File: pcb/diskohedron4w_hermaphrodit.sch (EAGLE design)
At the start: 23 parts, among them IC1 LM2596, U1 SN65LVDS047D, X1 87758-1216, X2 87758-1216

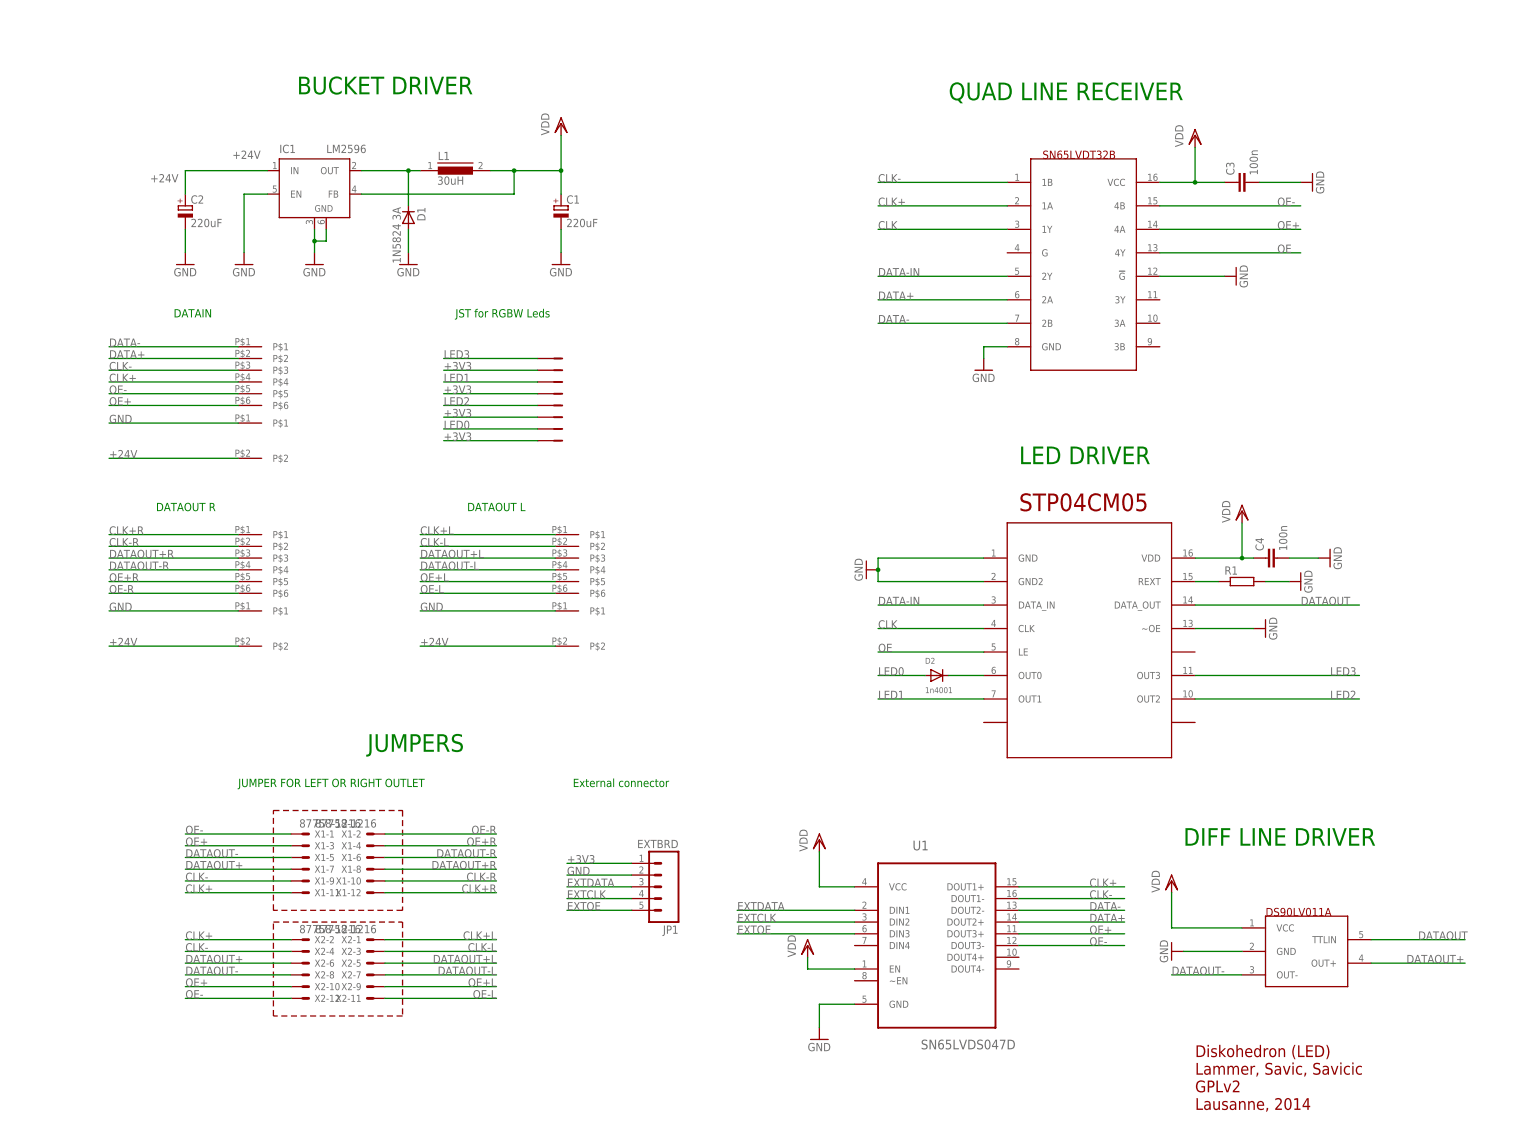
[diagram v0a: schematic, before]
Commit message: last commit before changing physical dimension
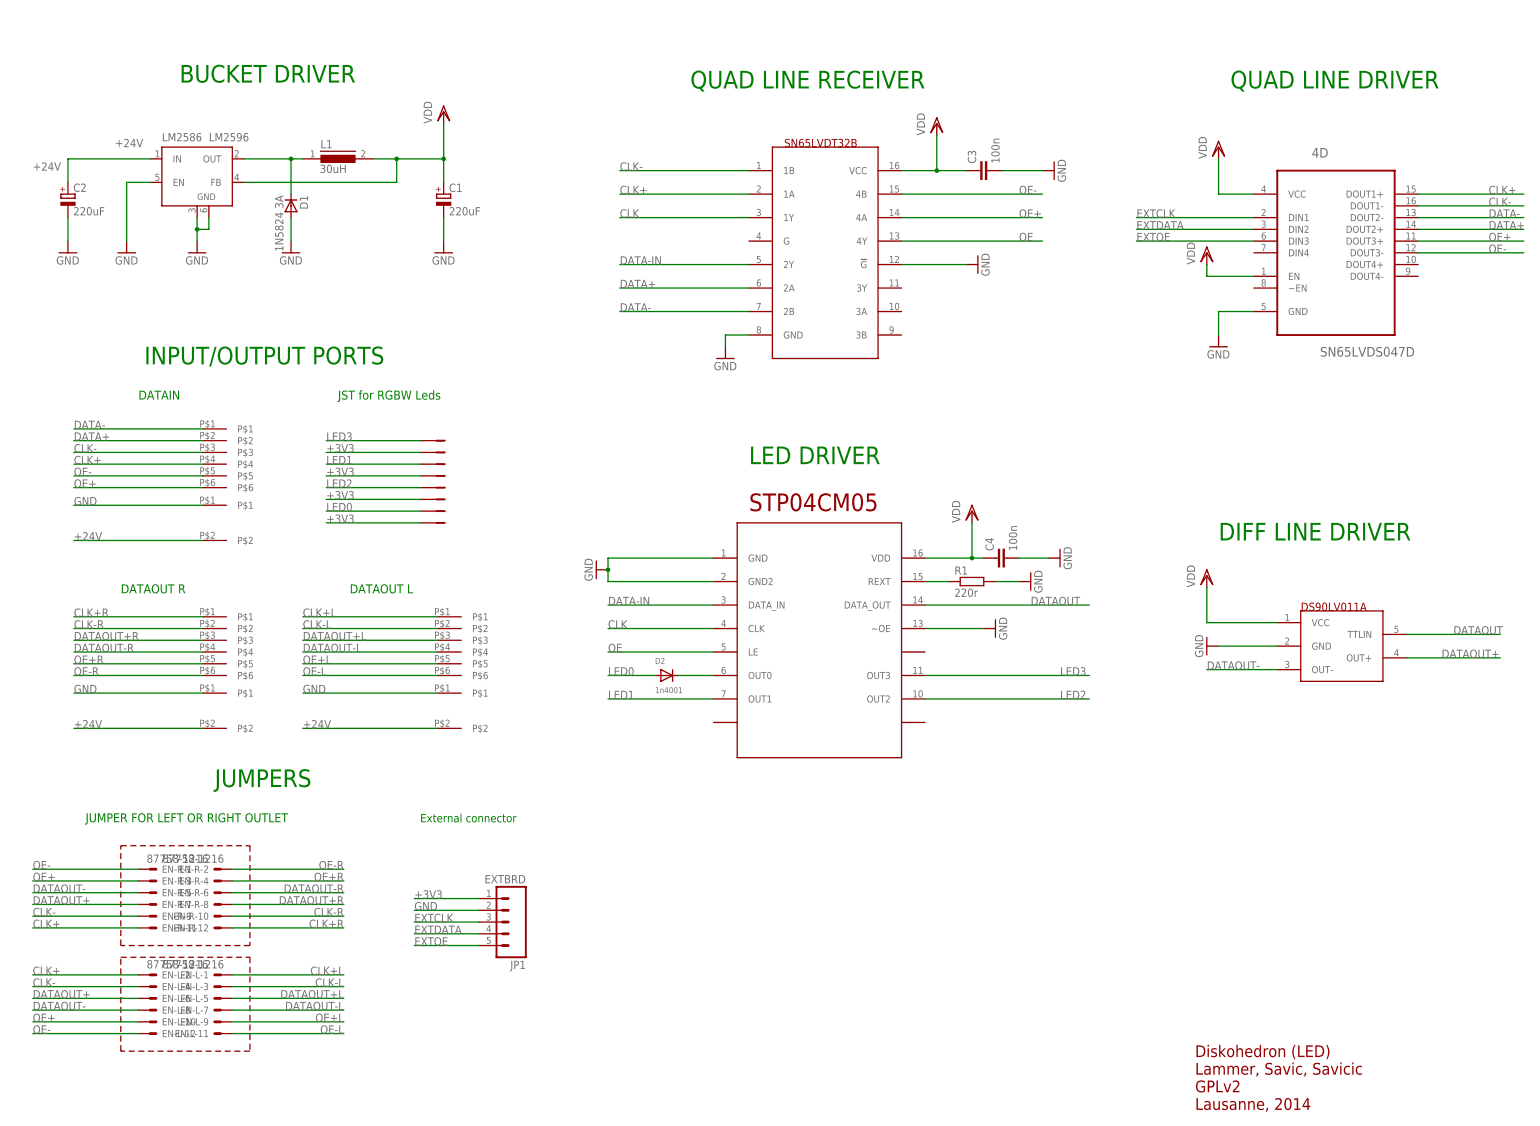
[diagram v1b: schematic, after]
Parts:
- removed IC1: LM2596, linear:LM2596S
- removed U$1: STP04CM05, stp04:STP04CM05
- removed U$11, U$5, U$8: HERMAPHRODITMINI6PIN, diskohedron:HERMAPHRODITMINI6PIN
- removed U$2: SN65LVDST32, diskohedron:SN65LVDST32
- removed U$3: DS90LV011A, diskohedron:DS90LV011A
- removed U$4: 8PIN-ZH, diskohedron:8PIN-ZH
- removed U1: SN65LVDS047D, Texas Instruments_By_element14_Batch_1:SN65LVDS047D
- removed X1, X2: 87758-1216, con-molex:87758-1216
- added 1D: DS90LV011A, diskohedron:DS90LV011A
- added 4D: SN65LVDS047D, Texas Instruments_By_element14_Batch_1:SN65LVDS047D
- added 4R: SN65LVDST32, diskohedron:SN65LVDST32
- added EN-L, EN-R: 87758-1216, con-molex:87758-1216
- added IN1, OUT-L, OUT-R: HERMAPHRODITMINI6PIN, diskohedron:HERMAPHRODITMINI6PIN
- added JST: 8PIN-ZH, diskohedron:8PIN-ZH
- added LM2586: LM2596, linear:LM2596S
- added STP04: STP04CM05, stp04:STP04CM05
- R1: value (none) -> 220r
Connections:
- net +24V: now also LM2586.IN; no longer IC1.IN
- net +3V3: now also 1D.VCC, 4D.EN, 4D.VCC, 4R.VCC, JST2.1, JST4.1, JST6.1, JST8.1, LM2586.FB, STP04.VDD; no longer IC1.FB, U$1.VDD, U$2.VCC, U$3.VCC, U$42.1, U$44.1, U$46.1, U$48.1, U1.EN, U1.VCC
- net CLK: now also 4R.1Y, STP04.CLK; no longer U$1.CLK, U$2.1Y
- net CLK+: now also 4D.DOUT1+, 4R.1A, EN-L-2.S, EN-R-11.S, IN1.P$4; no longer U$2.1A, U$8.P$4, U1.DOUT1+, X1-11.S, X2-2.S
- net CLK+L: now also EN-L-1.S, OUT-L.P$1; no longer U$11.P$1, X2-1.S
- net CLK+R: now also EN-R-12.S, OUT-R.P$1; no longer U$5.P$1, X1-12.S
- net CLK-: now also 4D.DOUT1-, 4R.1B, EN-L-4.S, EN-R-9.S, IN1.P$3; no longer U$2.1B, U$8.P$3, U1.DOUT1-, X1-9.S, X2-4.S
- net CLK-L: now also EN-L-3.S, OUT-L.P$2; no longer U$11.P$2, X2-3.S
- net CLK-R: now also EN-R-10.S, OUT-R.P$2; no longer U$5.P$2, X1-10.S
- net DATA+: now also 4D.DOUT2+, 4R.2A, IN1.P$2; no longer U$2.2A, U$8.P$2, U1.DOUT2+
- net DATA-: now also 4D.DOUT2-, 4R.2B, IN1.P$1; no longer U$2.2B, U$8.P$1, U1.DOUT2-
- net DATA-IN: now also 4R.2Y, STP04.DATA_IN; no longer U$1.DATA_IN, U$2.2Y
- net DATAOUT: now also 1D.TTLIN, STP04.DATA_OUT; no longer U$1.DATA_OUT, U$3.TTLIN
- net DATAOUT+: now also 1D.OUT+, EN-L-6.S, EN-R-7.S; no longer U$3.OUT+, X1-7.S, X2-6.S
- net DATAOUT+L: now also EN-L-5.S, OUT-L.P$3; no longer U$11.P$3, X2-5.S
- net DATAOUT+R: now also EN-R-8.S, OUT-R.P$3; no longer U$5.P$3, X1-8.S
- net DATAOUT-: now also 1D.OUT-, EN-L-8.S, EN-R-5.S; no longer U$3.OUT-, X1-5.S, X2-8.S
- net DATAOUT-L: now also EN-L-7.S, OUT-L.P$4; no longer U$11.P$4, X2-7.S
- net DATAOUT-R: now also EN-R-6.S, OUT-R.P$4; no longer U$5.P$4, X1-6.S
- net EXTCLK: now also 4D.DIN1, JP1.3; no longer JP1.4, U1.DIN2
- net EXTDATA: now also 4D.DIN2, JP1.4; no longer JP1.3, U1.DIN1
- net EXTOE: now also 4D.DIN3; no longer U1.DIN3
- net GND: now also 1D.GND, 4D.GND, 4R.!G, 4R.GND, LM2586.EN, LM2586.GND, LM2586.GND@1, STP04.GND, STP04.GND2, STP04.~OE; no longer IC1.EN, IC1.GND, IC1.GND@1, U$1.GND, U$1.GND2, U$1.~OE, U$2.!G, U$2.GND, U$3.GND, U1.GND
- net LED0: now also JST7.1; no longer U$47.1
- net LED1: now also JST3.1, STP04.OUT1; no longer U$1.OUT1, U$43.1
- net LED2: now also JST5.1, STP04.OUT2; no longer U$1.OUT2, U$45.1
- net LED3: now also JST1.1, STP04.OUT3; no longer U$1.OUT3, U$41.1
- net N$1: now also STP04.REXT; no longer U$1.REXT
- net N$2: now also LM2586.OUT; no longer IC1.OUT
- net N$3: now also STP04.OUT0; no longer U$1.OUT0
- net OE: now also 4R.4Y, STP04.LE; no longer U$1.LE, U$2.4Y
- net OE+: now also 4D.DOUT3+, 4R.4A, EN-L-10.S, EN-R-3.S, IN1.P$6; no longer U$2.4A, U$8.P$6, U1.DOUT3+, X1-3.S, X2-10.S
- net OE+L: now also EN-L-9.S, OUT-L.P$5; no longer U$11.P$5, X2-9.S
- net OE+R: now also EN-R-4.S, OUT-R.P$5; no longer U$5.P$5, X1-4.S
- net OE-: now also 4D.DOUT3-, 4R.4B, EN-L-12.S, EN-R-1.S, IN1.P$5; no longer U$2.4B, U$8.P$5, U1.DOUT3-, X1-1.S, X2-12.S
- net OE-L: now also EN-L-11.S, OUT-L.P$6; no longer U$11.P$6, X2-11.S
- net OE-R: now also EN-R-2.S, OUT-R.P$6; no longer U$5.P$6, X1-2.S
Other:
- note added: "INPUT/OUTPUT PORTS"
- note added: "QUAD LINE DRIVER"
- moved on the sheet: C1, C2, C3, C4, D1, D2, JP1, L1, R1

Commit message: order for itead 12/05/2014 #100029337
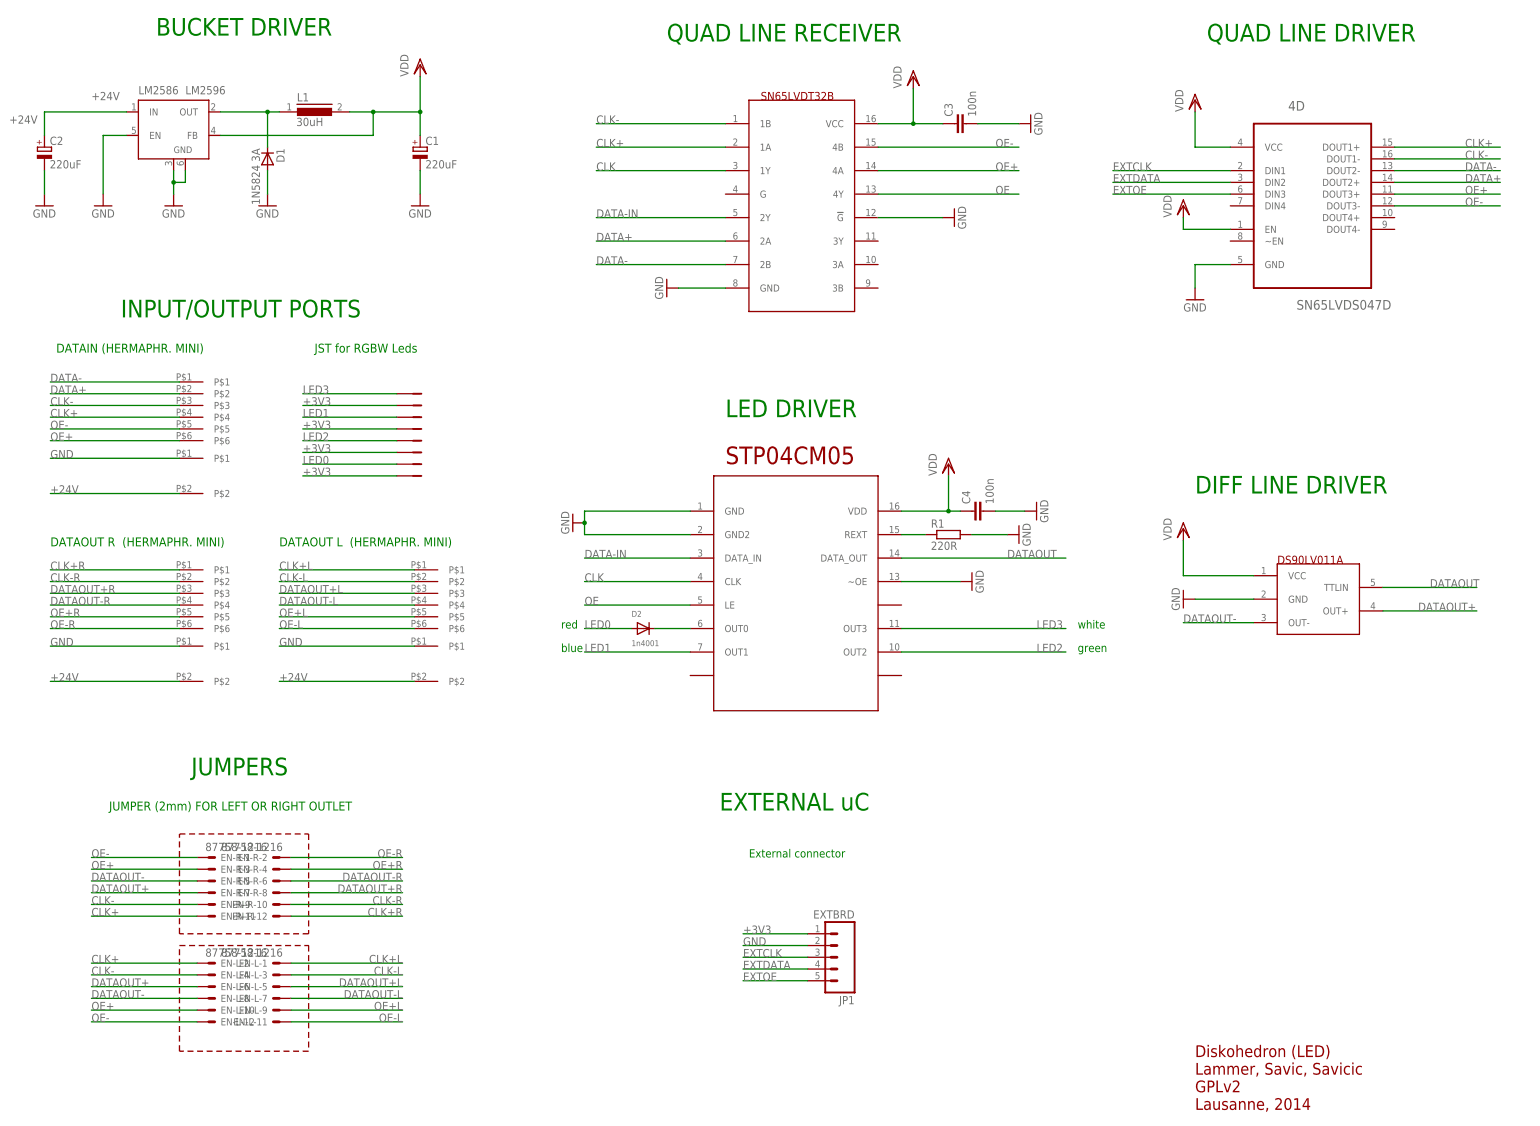
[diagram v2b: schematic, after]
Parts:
- R1: value 220r -> 220R
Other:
- note added: "DATAIN (HERMAPHR. MINI)"
- note added: "DATAOUT L (HERMAPHR. MINI)"
- note added: "DATAOUT R (HERMAPHR. MINI)"
- note added: "EXTERNAL uC"
- note added: "JUMPER (2mm) FOR LEFT OR RIGHT OUTLET"
- note added: "blue"
- note added: "green"
- note added: "red"
- note added: "white"
- note removed: "DATAIN"
- note removed: "DATAOUT L"
- note removed: "DATAOUT R"
- note removed: "JUMPER FOR LEFT OR RIGHT OUTLET"
- moved on the sheet: 4D, C1, C2, C3, C4, D1, D2, EN-L-1, EN-L-10, EN-L-11, EN-L-12, EN-L-2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
